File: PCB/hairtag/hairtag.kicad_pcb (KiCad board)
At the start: 2 copper layers, 19 parts, among them J1 Flash, J2 BAT, U1 ESP32-C3FH4, U2 HT7533-1_C14289, X1 XL2EL89CPI-111YLC-40M

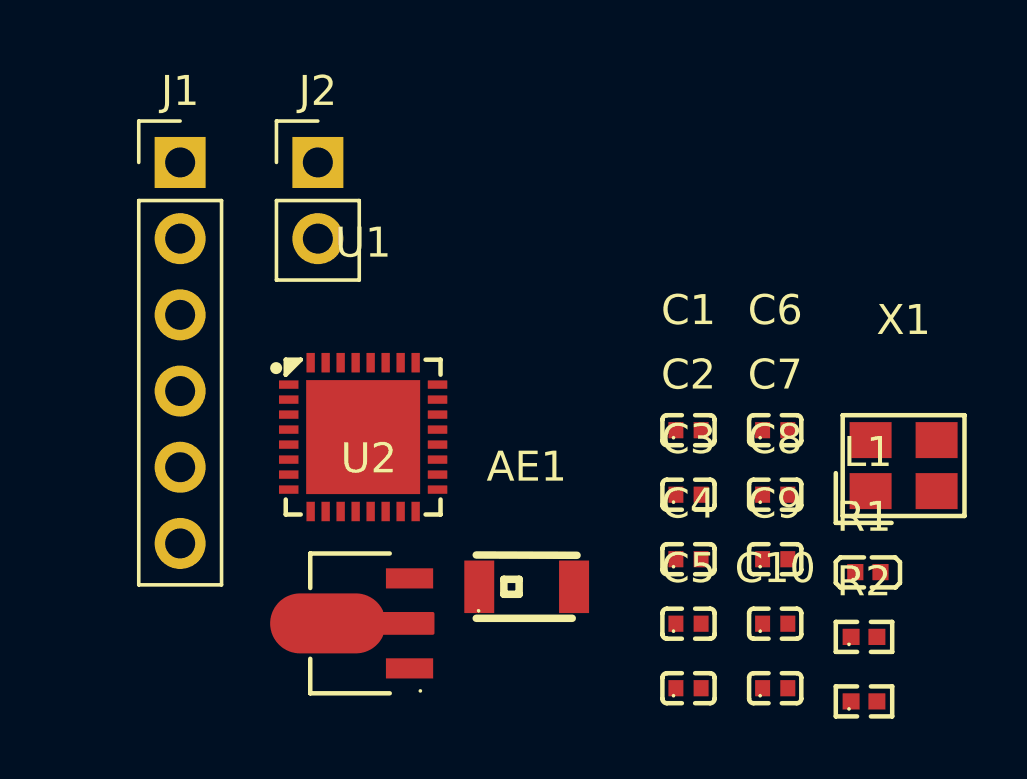
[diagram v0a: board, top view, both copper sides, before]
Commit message: asdf
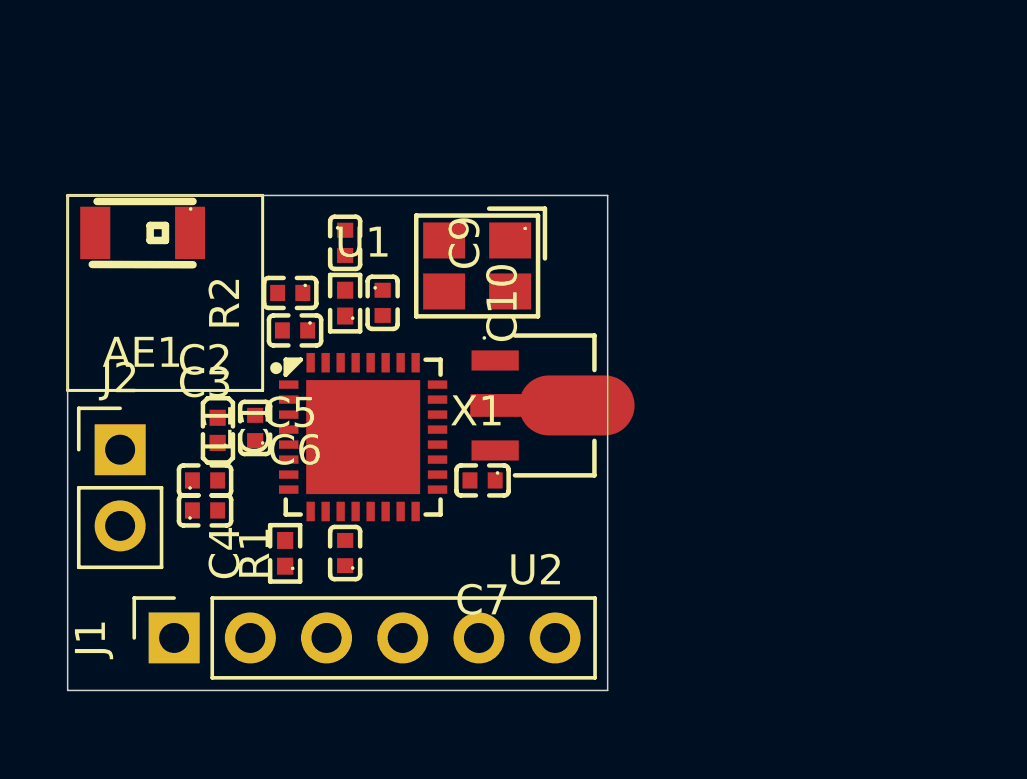
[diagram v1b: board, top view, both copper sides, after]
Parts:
- removed C8: 1uF, lcsc:C0402
- J1: footprint Connector_PinHeader_2.54mm:PinHeader_1x06_P2.54mm_Vertical -> Connector_PinSocket_2.54mm:PinSocket_1x06_P2.54mm_Vertical
- moved L1 22.2 mm to (53.2, 54.8), turned to 90 degrees
- moved R2 21.8 mm to (57.5, 50.6), turned to 90 degrees
- moved R1 19.5 mm to (55.5, 58.9), turned to 90 degrees
- moved C9 19.1 mm to (57.5, 48.6), turned to -90 degrees
- moved C5 18.7 mm to (55.7, 50.2), turned to 180 degrees
- moved C10 18.3 mm to (58.8, 50.6), turned to -90 degrees
- moved AE1 17.4 mm to (50.8, 48.2), turned to 180 degrees
- moved C6 16.3 mm to (55.8, 51.5), turned to 180 degrees
- moved C3 16.2 mm to (52.8, 57.5)
- moved C2 16.1 mm to (52.8, 56.5)
- moved J1 15.9 mm to (51.8, 61.8), turned to 90 degrees
- moved X1 15.7 mm to (61.9, 49.4), turned to 180 degrees
- moved C1 14.4 mm to (54.5, 54.8), turned to 90 degrees
- moved C4 11.7 mm to (57.5, 58.9), turned to 90 degrees
- moved J2 11.6 mm to (50.0, 55.5)
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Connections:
- C1 pad 1: Net-(C1-Pad1) -> GND
- C1 pad 2: GND -> Net-(C1-Pad2)
- C2 pad 2: GND -> /VCC
- C3 pad 2: GND -> /VCC
- C4 pad 2: GND -> /VCC
- C5 pad 1: GND -> /VCC
- C6 pad 1: GND -> /VCC
- C7 pad 2: GND -> /VCC
- J1 pad 1: GND -> /VCC
- L1 pad 1: GND -> /VCC
- L1 pad 2: Net-(C1-Pad1) -> Net-(C1-Pad2)
- U1 pad 11: GND -> /VCC
- U1 pad 17: GND -> /VCC
- U1 pad 2: Net-(C1-Pad1) -> Net-(C1-Pad2)
- U1 pad 3: Net-(C1-Pad1) -> Net-(C1-Pad2)
- U1 pad 31: GND -> /VCC
- U1 pad 32: GND -> /VCC
- U2 pad 3: GND -> /VCC
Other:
- board outline added: 18 x 16.5 mm
